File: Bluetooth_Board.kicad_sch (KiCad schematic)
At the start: 62 parts, among them IC1 STM32WB55CGU6, J1 5V Power Pins, J10 LPUART1_Header, J11 3V3 Power Pins, J12 Pin_Header, J13 3V3 Power Source Jumpers, J14 Debug_Pins, J15 USART1_Header, J19 Power Select Jumpers, J2 SMA PCB END LAUNCH JACK ROUND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, J20 SPI1_Header, J3 User Button Jumper, J4 Coin Battery Jumper, J5 Power Pins, J6 USB_B_Micro, J7 I2C3_Header, J8 BOOT0_Jumper, J9 I2C1_Header, U3 USBLC6-2SC6, Y3 Clock_ECS-327MVATX-7-CN-TR, Y4 ABM3B-32.000MHZ-8-R30-B1U-T

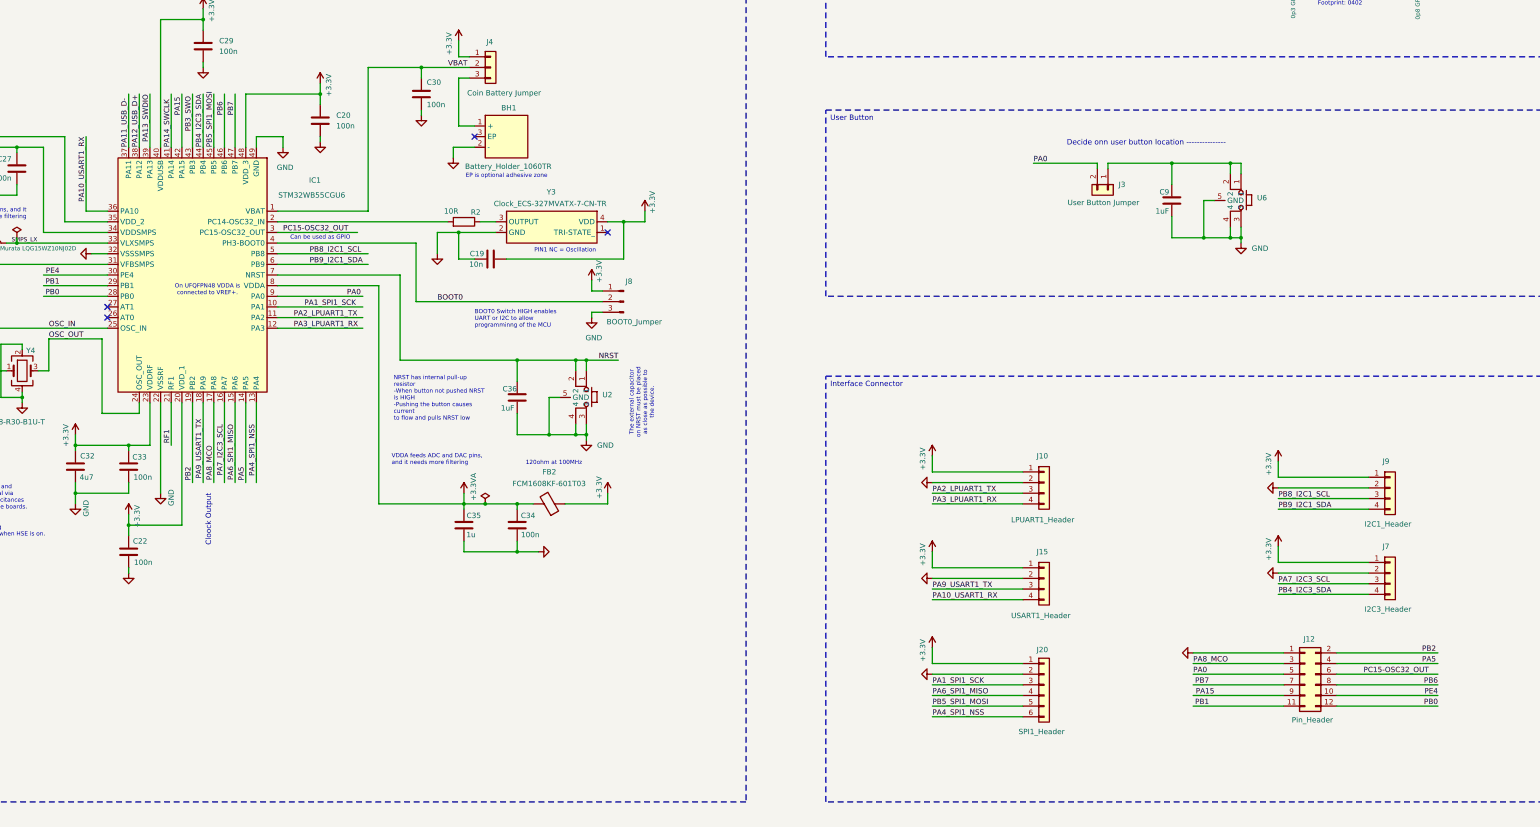
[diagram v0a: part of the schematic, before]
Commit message: Update
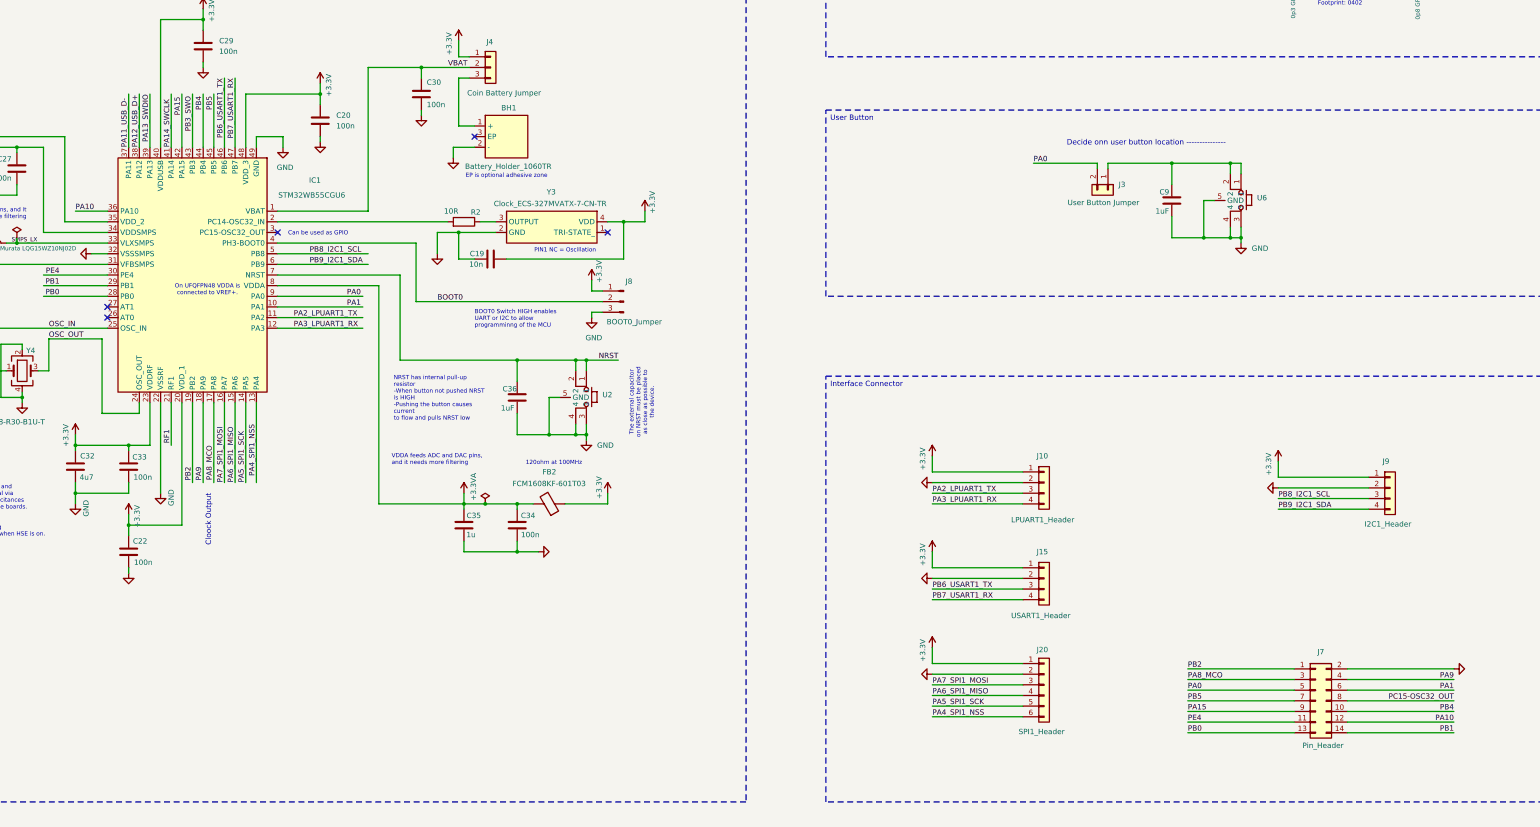
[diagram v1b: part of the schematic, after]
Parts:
- removed J12: Pin_Header, Connector_PinHeader_2.54mm:PinHeader_2x06_P2.54mm_Vertical, symbol Connector_Generic:Conn_02x06_Odd_Even
- removed J7: I2C3_Header, Connector_PinHeader_2.54mm:PinHeader_1x04_P2.54mm_Vertical, symbol Connector_Generic:Conn_01x04
- added J7: Pin_Header, Connector_PinHeader_2.54mm:PinHeader_2x07_P2.54mm_Vertical, symbol Connector_Generic:Conn_02x07_Odd_Even
- R2, R6: footprint Resistor_SMD:R_0805_2012Metric_Pad1.20x1.40mm_HandSolder -> Resistor_SMD:R_0603_1608Metric_Pad0.98x0.95mm_HandSolder
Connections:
- net GND: now also J7.2 (Pin_2)
- net PA0: now also J7.5 (Pin_5)
- net PA15: now also J7.9 (Pin_9)
- net PA8_MCO: now also J7.3 (Pin_3)
- net PB0: now also J7.13 (Pin_13)
- net PB1: now also J7.14 (Pin_14)
- net PB2: now also J7.1 (Pin_1)
- net PC15-OSC32_OUT: now also J7.8 (Pin_8); no longer IC1.3 (PC15-OSC32_OUT)
- net PE4: now also J7.11 (Pin_11)
- net PA10_USART1_RX renamed PA10
- net PA10: now also J7.12 (Pin_12); no longer J15.4 (Pin_4)
- net PA1_SPI1_SCK renamed PA1
- net PA1: now also J7.6 (Pin_6); no longer J20.3 (Pin_3)
- net PA5 renamed PA5_SPI1_SCK
- net PA5_SPI1_SCK: now also J20.5 (Pin_5)
- net PA7_I2C3_SCL renamed PA7_SPI1_MOSI
- net PA7_SPI1_MOSI: now also J20.3 (Pin_3)
- net PA9_USART1_TX renamed PA9
- net PA9: now also J7.4 (Pin_4); no longer J15.3 (Pin_3)
- net PB4_I2C3_SDA renamed PB4
- net PB4: now also J7.10 (Pin_10)
- net PB5_SPI1_MOSI renamed PB5
- net PB5: now also J7.7 (Pin_7); no longer J20.5 (Pin_5)
- net PB6 renamed PB6_USART1_TX
- net PB6_USART1_TX: now also J15.3 (Pin_3)
- net PB7 renamed PB7_USART1_RX
- net PB7_USART1_RX: now also J15.4 (Pin_4)
- no-connect marks 6 -> 7
